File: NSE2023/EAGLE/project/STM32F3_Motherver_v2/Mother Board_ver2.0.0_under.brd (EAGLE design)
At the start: 50 x 35 mm, 6 parts

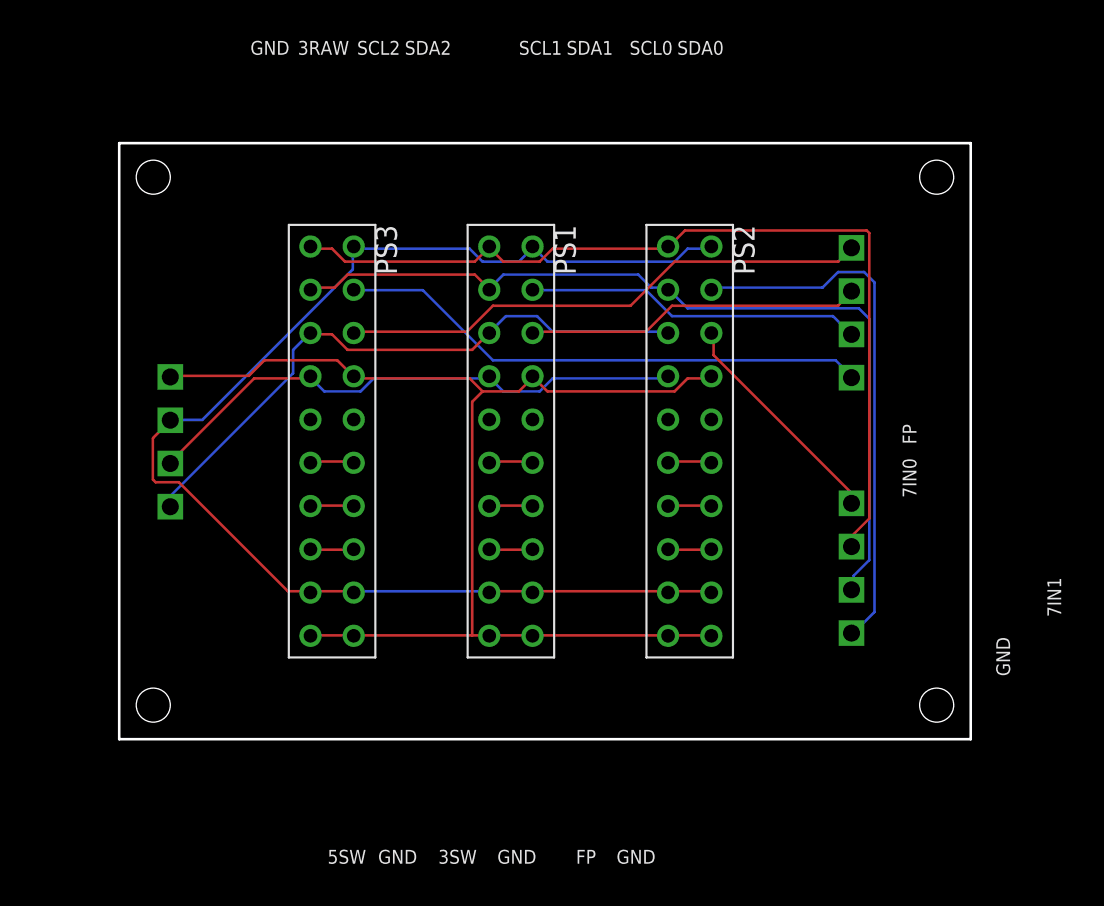
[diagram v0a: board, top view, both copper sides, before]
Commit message: create final board
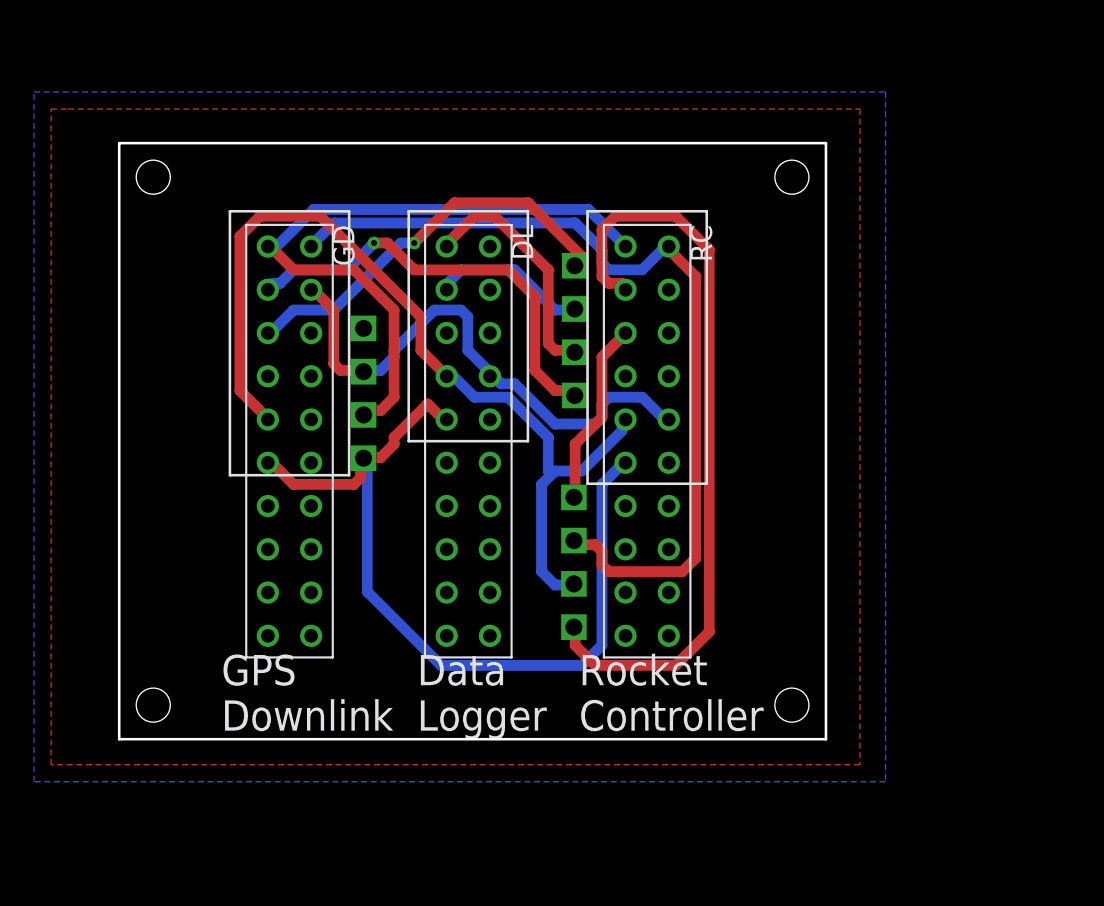
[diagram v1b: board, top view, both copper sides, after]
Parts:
- removed CON5, CON6: (no value), Connector:2.5_MINI-SPOX_4PIN
- removed PS1, PS2, PS3: (no value), PinSocket:2X10
- added DL, GD, RC: (no value), PinSocket:2X10
- added POWER, SENSER-MOTOR: (no value), Connector:2.5_MINI-SPOX_4PIN
- moved CON7 16.3 mm to (26.8, 21.4)
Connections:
- removed net SWCLK0: PS2.P$5, PS2.P$6
- removed net SWCLK1: PS1.P$5, PS1.P$6
- removed net SWCLK2: PS3.P$5, PS3.P$6
- removed net SWDIO0: PS2.P$7, PS2.P$8
- removed net SWDIO1: PS1.P$7, PS1.P$8
- removed net SWDIO2: PS3.P$7, PS3.P$8
- removed net SWO0: PS2.P$10, PS2.P$9
- removed net SWO1: PS1.P$10, PS1.P$9
- removed net SWO2: PS3.P$10, PS3.P$9
- new net NRST0: RC.P$14
- new net NRST1: DL.P$16
- new net NRST2: GD.P$14
- net +3V3: now also DL.P$13, GD.P$17, POWER.P$3, RC.P$11; no longer CON5.P$3, PS1.P$19, PS1.P$3, PS1.P$4, PS2.P$19, PS2.P$3, PS2.P$4, PS3.P$19, PS3.P$3, PS3.P$4
- net +5V: now also GD.P$20, POWER.P$4, RC.P$20; no longer CON5.P$4, PS1.P$14, PS2.P$14, PS3.P$14
- net FPRAW: now also DL.P$12, GD.P$10, POWER.P$2, RC.P$10; no longer CON5.P$2, PS1.P$16, PS2.P$16, PS3.P$16
- net GND: now also DL.P$11, GD.P$9, POWER.P$1, RC.P$9; no longer CON5.P$1, PS1.P$1, PS1.P$13, PS1.P$2, PS2.P$1, PS2.P$13, PS2.P$2, PS3.P$1, PS3.P$13, PS3.P$2
- net PWM: now also GD.P$19, RC.P$19, SENSER-MOTOR.P$4; no longer CON6.P$4, PS1.P$20, PS2.P$20, PS3.P$20
- net SCL0: now also RC.P$16, SENSER-MOTOR.P$2; no longer CON6.P$2, PS2.P$15
- net SCL1: now also DL.P$18; no longer PS1.P$15
- net SCL2: now also GD.P$16; no longer PS3.P$15
- net SDA0: now also RC.P$18, SENSER-MOTOR.P$1; no longer CON6.P$1, PS2.P$17
- net SDA1: now also DL.P$20; no longer PS1.P$17
- net SDA2: now also GD.P$18; no longer PS3.P$17
- net SW: now also DL.P$14, GD.P$12, RC.P$12, SENSER-MOTOR.P$3; no longer CON6.P$3, PS1.P$18, PS2.P$18, PS3.P$18
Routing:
- net GND: track 72.3 -> 0.00 mm
- net +3V3: track 78.1 -> 32.2 mm
- net SDA0: track 31.5 -> 44.7 mm
- net FPRAW: track 36.3 -> 49.4 mm
- net SCL1: track 19.8 -> 9.16 mm
- net SCL2: track 31.3 -> 24.1 mm, vias 0 -> 1
- net +5V: track 33.0 -> 39.2 mm
- net SDA2: track 31.4 -> 25.4 mm, vias 0 -> 1
- net SDA1: track 19.8 -> 14.1 mm
- net SWO0: track 2.63 -> 0.00 mm
- net SWO1: track 2.62 -> 0.00 mm
- net SWO2: track 2.62 -> 0.00 mm
- net SWDIO0: track 2.56 -> 0.00 mm
- net SCL0: track 13.4 -> 10.9 mm
- net SWCLK0: track 2.55 -> 0.00 mm
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- added copper zone on layer 1, net GND
- added copper zone on layer 16, net GND
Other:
- board size 50 x 35 mm -> 41.5 x 35 mm
- board text added: "Data Logger"
- board text added: "GPS Downlink"
- board text added: "Rocket Controller"
- board text removed: "3RAW"
- board text removed: "3SW"
- board text removed: "5SW"
- board text removed: "7IN0"
- board text removed: "7IN1"
- board text removed: "FP"
- board text removed: "GND"
- board text removed: "SCL0"
- board text removed: "SCL1"
- board text removed: "SCL2"
- board text removed: "SDA0"
- board text removed: "SDA1"
- board text removed: "SDA2"
